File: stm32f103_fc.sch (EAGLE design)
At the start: 37 parts, among them IC1 STM32F10XCXT6, U1 RT9193-33GB, Y1 8MHz, Y2 32.768MHz

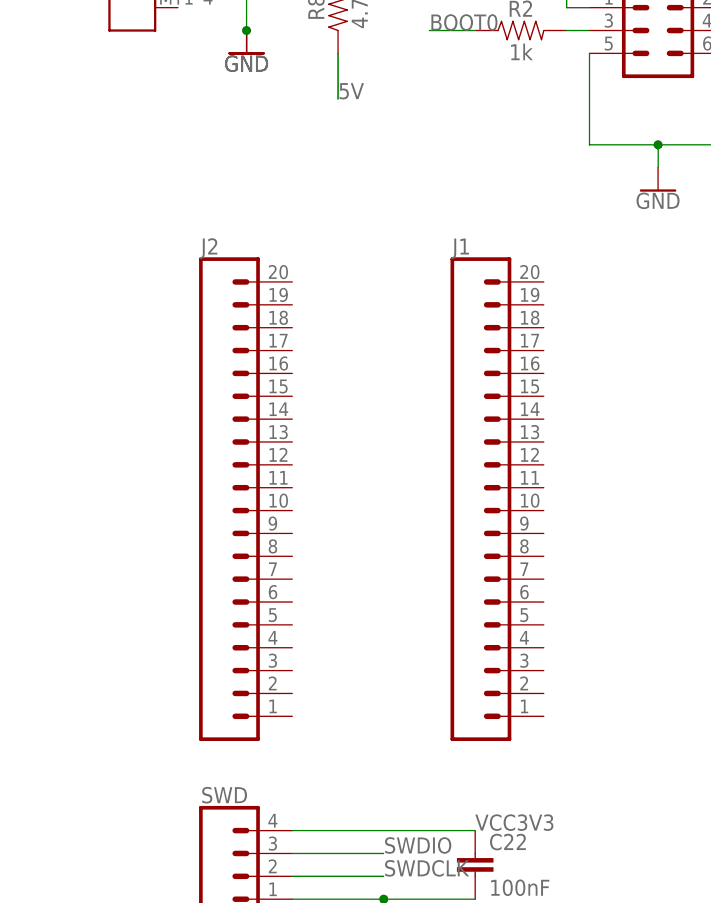
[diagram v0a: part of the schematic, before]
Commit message: added more lable
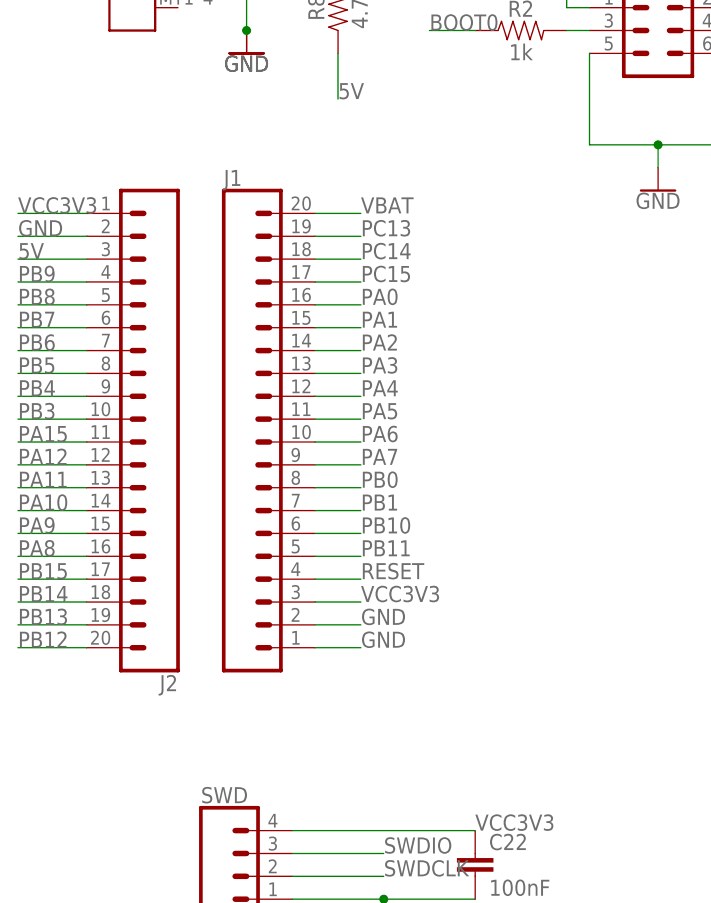
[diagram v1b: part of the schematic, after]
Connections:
- net 5V: now also J2.3
- net GND: now also J1.1, J1.2, J2.2
- net PA0: now also J1.16
- net PA1: now also J1.15
- net PA10: now also J2.14
- net PA11: now also J2.13
- net PA12: now also J2.12
- net PA15: now also J2.11
- net PA2: now also J1.14
- net PA3: now also J1.13
- net PA4: now also J1.12
- net PA5: now also J1.11
- net PA6: now also J1.10
- net PA7: now also J1.9
- net PA8: now also J2.16
- net PA9: now also J2.15
- net PB0: now also J1.8
- net PB1: now also J1.7
- net PB10: now also J1.6
- net PB11: now also J1.5
- net PB12: now also J2.20
- net PB13: now also J2.19
- net PB14: now also J2.18
- net PB15: now also J2.17
- net PB3: now also J2.10
- net PB4: now also J2.9
- net PB5: now also J2.8
- net PB6: now also J2.7
- net PB7: now also J2.6
- net PB8: now also J2.5
- net PB9: now also J2.4
- net PC13: now also J1.19
- net PC14: now also J1.18
- net PC15: now also J1.17
- net RESET: now also J1.4
- net VBAT: now also J1.20
- net VCC3V3: now also J1.3, J2.1
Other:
- moved on the sheet: J1, J2
